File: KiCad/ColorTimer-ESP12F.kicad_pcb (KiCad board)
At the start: 2 copper layers, 1 part, among them U1 ESP-12F

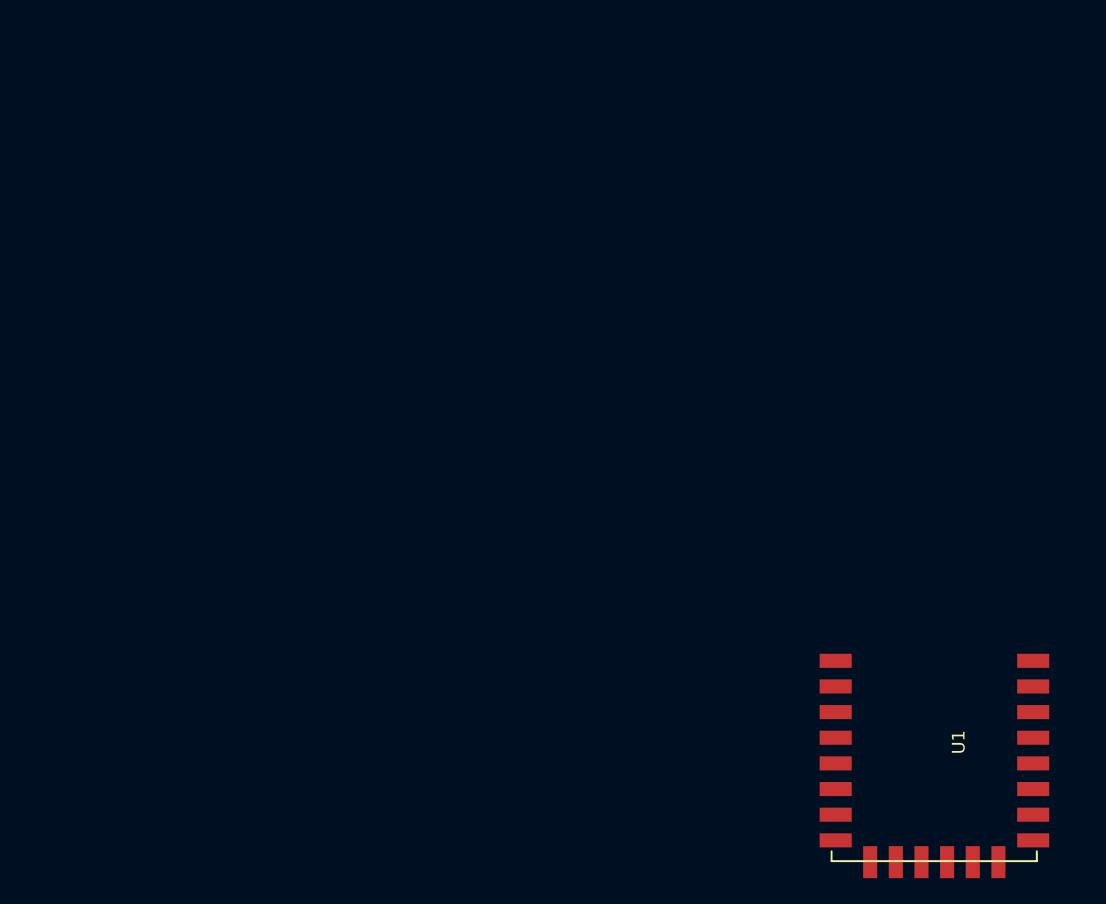
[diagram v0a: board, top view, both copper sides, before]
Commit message: 回路図、パターン暫定版
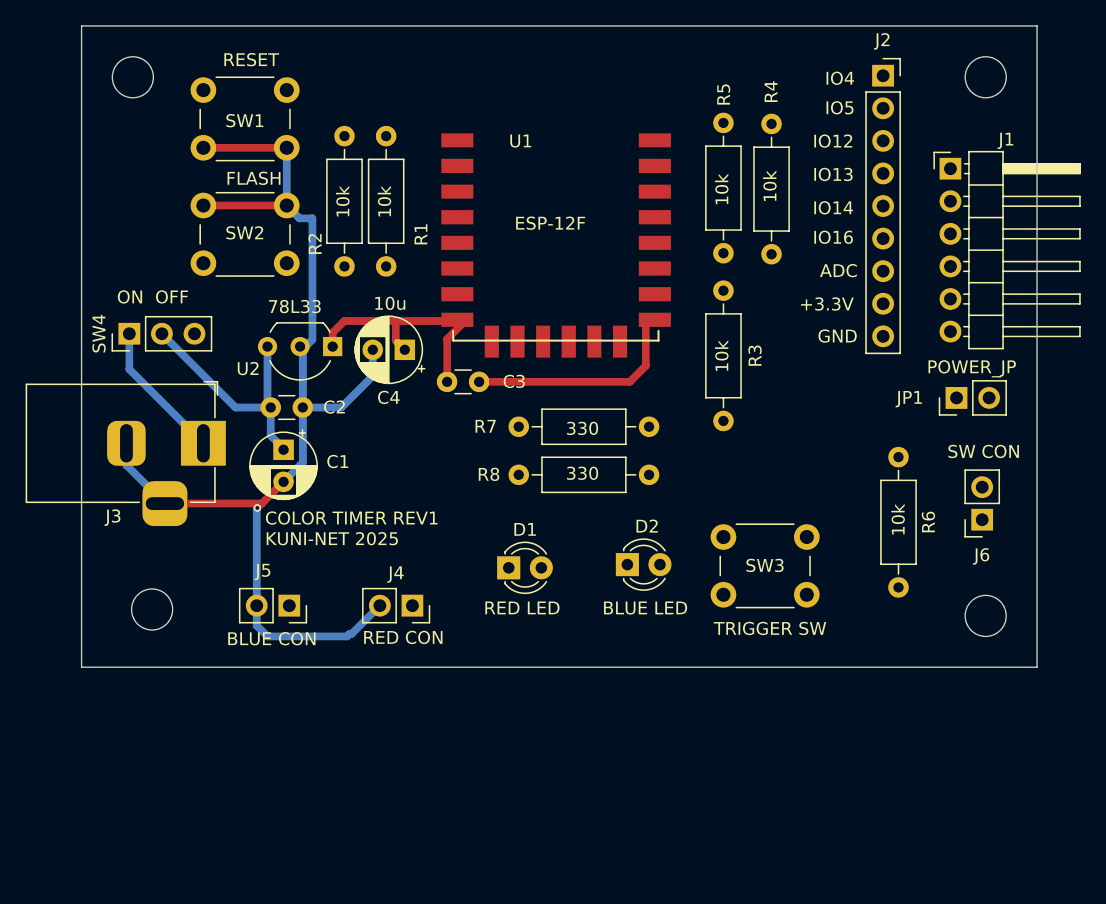
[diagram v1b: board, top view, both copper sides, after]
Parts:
- added C1: 100u, Capacitor_THT:CP_Radial_D5.0mm_P2.50mm, F.Cu at (110.8, 73.0)
- added C2: 0.1u, Capacitor_THT:C_Disc_D3.0mm_W1.6mm_P2.50mm, F.Cu at (109.8, 69.8)
- added C3: 0.1u, Capacitor_THT:C_Disc_D3.0mm_W1.6mm_P2.50mm, F.Cu at (123.5, 67.8)
- added C4: 10u, Capacitor_THT:CP_Radial_D5.0mm_P2.50mm, F.Cu at (120.2, 65.2)
- added D1: RED LED, LED_THT:LED_D3.0mm, F.Cu at (128.3, 82.2)
- added D2: BLUE LED, LED_THT:LED_D3.0mm, F.Cu at (137.6, 82.0)
- added H1: MountingHole, MountingHole:MountingHole_3.2mm_M3, F.Cu at (99.0, 44.0)
- added H2: MountingHole, MountingHole:MountingHole_3.2mm_M3, F.Cu at (100.5, 85.5)
- added H3: MountingHole, MountingHole:MountingHole_3.2mm_M3, F.Cu at (165.5, 44.0)
- added H4: MountingHole, MountingHole:MountingHole_3.2mm_M3, F.Cu at (165.5, 86.0)
- added J1: SERIAL CON, Connector_PinHeader_2.54mm:PinHeader_1x06_P2.54mm_Horizontal, F.Cu at (162.8, 51.1)
- added J2: GPIO_CON, Connector_PinSocket_2.54mm:PinSocket_1x09_P2.54mm_Vertical, F.Cu at (157.5, 43.9)
- added J3: Barrel_Jack_Switch, Connector_BarrelJack:BarrelJack_Horizontal, F.Cu at (104.5, 72.5)
- added J4: RED_CON, Connector_PinSocket_2.54mm:PinSocket_1x02_P2.54mm_Vertical, F.Cu at (120.8, 85.2)
- added J5: BLUE_CON, Connector_PinSocket_2.54mm:PinSocket_1x02_P2.54mm_Vertical, F.Cu at (111.2, 85.2)
- added J6: SW_CON, Connector_PinSocket_2.54mm:PinSocket_1x02_P2.54mm_Vertical, F.Cu at (165.2, 78.5)
- added JP1: Power JP, Connector_PinHeader_2.54mm:PinHeader_1x02_P2.54mm_Vertical, F.Cu at (163.2, 69.0)
- added R1: 10k, Resistor_THT:R_Axial_DIN0207_L6.3mm_D2.5mm_P10.16mm_Horizontal, F.Cu at (118.8, 58.8)
- added R2: 10k, Resistor_THT:R_Axial_DIN0207_L6.3mm_D2.5mm_P10.16mm_Horizontal, F.Cu at (115.5, 58.8)
- added R3: 10k, Resistor_THT:R_Axial_DIN0207_L6.3mm_D2.5mm_P10.16mm_Horizontal, F.Cu at (145.1, 60.6)
- added R4: 10k, Resistor_THT:R_Axial_DIN0207_L6.3mm_D2.5mm_P10.16mm_Horizontal, F.Cu at (148.8, 57.8)
- added R5: 10k, Resistor_THT:R_Axial_DIN0207_L6.3mm_D2.5mm_P10.16mm_Horizontal, F.Cu at (145.1, 57.7)
- added R6: 10k, Resistor_THT:R_Axial_DIN0207_L6.3mm_D2.5mm_P10.16mm_Horizontal, F.Cu at (158.7, 73.6)
- added R7: 330, Resistor_THT:R_Axial_DIN0207_L6.3mm_D2.5mm_P10.16mm_Horizontal, F.Cu at (139.2, 71.2)
- added R8: 330, Resistor_THT:R_Axial_DIN0207_L6.3mm_D2.5mm_P10.16mm_Horizontal, F.Cu at (139.2, 75.0)
- added SW1: RESET, Button_Switch_THT:SW_PUSH_6mm_H8mm, F.Cu at (111.0, 49.5)
- added SW2: FLASH, Button_Switch_THT:SW_PUSH_6mm_H8mm, F.Cu at (111.0, 58.5)
- added SW3: Trigger SW, Button_Switch_THT:SW_PUSH_6mm_H8mm, F.Cu at (145.1, 79.8)
- added SW4: POWER_SW, Connector_PinHeader_2.54mm:PinHeader_1x03_P2.54mm_Vertical, F.Cu at (98.7, 64.0)
- added U2: L78L33_TO92, Package_TO_SOT_THT:TO-92_Inline_Wide, F.Cu at (114.6, 65.0)
- moved U1 50.2 mm to (125.0, 48.9)
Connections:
- U1 pad 1: unconnected-(U1-REST-Pad1) -> Net-(U1-REST)
- U1 pad 10: unconnected-(U1-GPIO15-Pad10) -> Net-(U1-GPIO15)
- U1 pad 11: unconnected-(U1-GPIO2-Pad11) -> Net-(U1-GPIO2)
- U1 pad 12: unconnected-(U1-GPIO0-Pad12) -> Net-(U1-GPIO0)
- U1 pad 13: unconnected-(U1-GPIO4-Pad13) -> /GPIO4
- U1 pad 14: unconnected-(U1-GPIO5-Pad14) -> /GPIO5
- U1 pad 15: unconnected-(U1-RXD-Pad15) -> Net-(J1-Pin_4)
- U1 pad 16: unconnected-(U1-TXD-Pad16) -> Net-(J1-Pin_5)
- U1 pad 2: unconnected-(U1-ADC-Pad2) -> /ADC
- U1 pad 3: unconnected-(U1-CH_PD-Pad3) -> Net-(U1-CH_PD)
- U1 pad 4: unconnected-(U1-GPIO16-Pad4) -> /GPIO16
- U1 pad 5: unconnected-(U1-GPIO14-Pad5) -> /GPIO14
- U1 pad 6: unconnected-(U1-GPIO12-Pad6) -> /GPIO12
- U1 pad 7: unconnected-(U1-GPIO13-Pad7) -> /GPIO13
- U1 pad 8: unconnected-(U1-VCC-Pad8) -> +3.3V
- U1 pad 9: unconnected-(U1-GND-Pad9) -> GND
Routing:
- net GND: track 0.00 -> 103.6 mm, vias 0 -> 1
- net +3.3V: track 0.00 -> 19.9 mm
- net Net-(SW4-B): track 0.00 -> 19.4 mm
- net Net-(SW4-A): track 0.00 -> 10.9 mm
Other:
- board outline added: 74.5 x 50 mm
- board text added: "+3.3V"
- board text added: "10k"
- board text added: "10u"
- board text added: "330"
- board text added: "78L33"
- board text added: "ADC"
- board text added: "BLUE CON"
- board text added: "BLUE LED"
- board text added: "COLOR TIMER REV1 KUNI-NET 2025"
- board text added: "ESP-12F"
- board text added: "FLASH"
- board text added: "GND"
- board text added: "IO12"
- board text added: "IO13"
- board text added: "IO14"
- board text added: "IO16"
- board text added: "IO4"
- board text added: "IO5"
- board text added: "ON OFF"
- board text added: "POWER_JP"
- board text added: "RED CON"
- board text added: "RED LED"
- board text added: "RESET"
- board text added: "SW CON"
- board text added: "TRIGGER SW"
